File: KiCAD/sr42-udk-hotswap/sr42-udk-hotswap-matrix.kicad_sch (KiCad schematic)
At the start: 44 parts

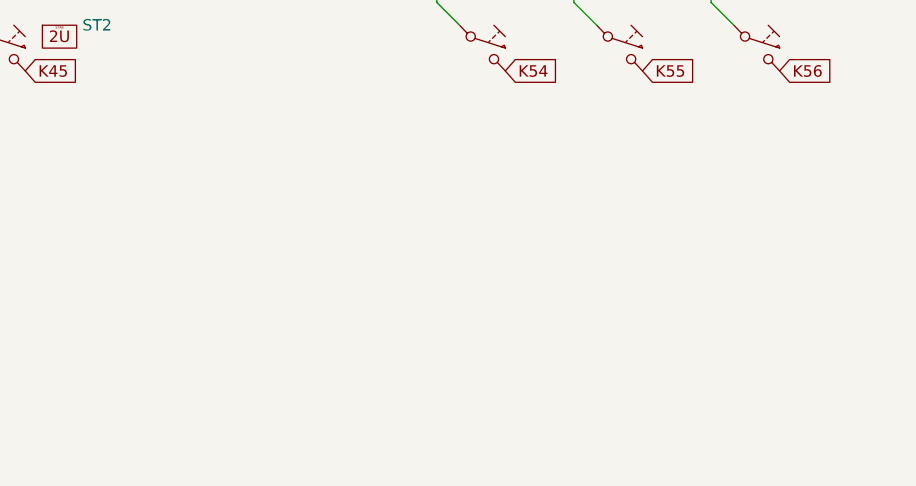
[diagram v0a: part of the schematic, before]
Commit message: wip-2025-11-24
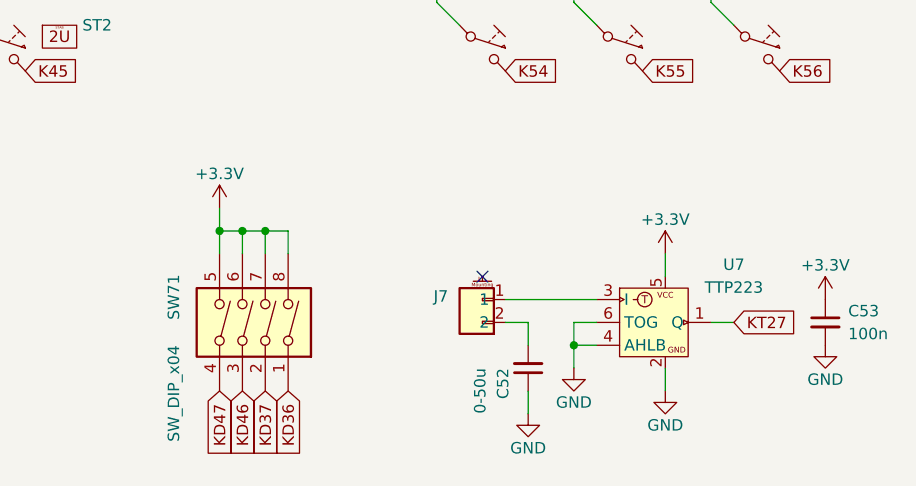
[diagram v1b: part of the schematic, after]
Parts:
- added C52: 0-50u, Capacitor_SMD:C_0603_1608Metric, symbol ts-kicad-lib:C
- added C53: 100n, Capacitor_SMD:C_0603_1608Metric, symbol ts-kicad-lib:C
- added J7: ~, Connector_JST:JST_SH_SM02B-SRSS-TB_1x02-1MP_P1.00mm_Horizontal, symbol ts-kicad-lib:CONN_02
- added SW71: SW_DIP_x04, ts-kicad-lib:SW_DIP_SPSTx04, symbol Switch:SW_DIP_x04
- added U7: TTP223, Package_TO_SOT_SMD:SOT-23-6_Handsoldering, symbol ts-kicad-lib:TTP223
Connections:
- net +3.3V: now also C53.1, SW71.5, SW71.6, SW71.7, SW71.8, U7.5 (VDD)
- new net: J7.1, U7.3 (I)
- new net: C52.2, J7.2
- new net GND: C52.1, C53.2, U7.2 (VSS), U7.4 (AHLB), U7.6 (TOG)
- new net KD36: SW71.1
- new net KD37: SW71.2
- new net KD46: SW71.3
- new net KD47: SW71.4
- new net KT27: U7.1 (Q)
- no-connect marks 0 -> 1
